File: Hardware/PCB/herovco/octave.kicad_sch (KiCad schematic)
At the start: 9 parts, among them SW1 SW_Rotary12

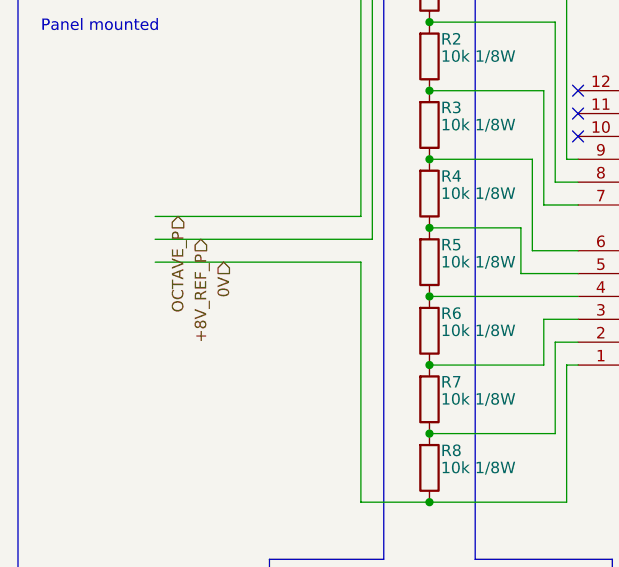
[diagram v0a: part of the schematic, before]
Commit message: Change pot symbols and fix orientation, other small tweaks
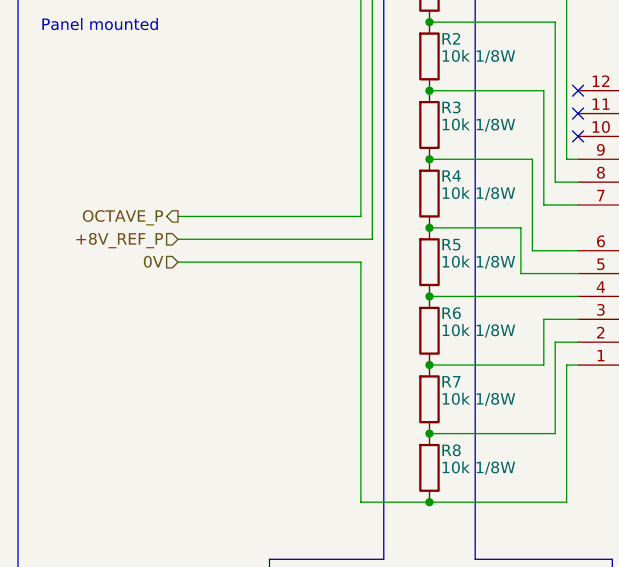
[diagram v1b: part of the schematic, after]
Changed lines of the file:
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@@
   (no_connect (at 147.32 82.55))
   (no_connect (at 147.32 77.47))
-  (wire (pts (xy 100.33 93.98) (xy 124.46 93.98))
+  (wire (pts (xy 102.87 93.98) (xy 124.46 93.98))
     (stroke (width 0) (type default) (color 0 0 0 0))
   )
@@
   )
   (polyline (pts (xy 125.73 129.54) (xy 113.03 129.54))
-    (stroke (width 0) (type default) (color 0 0 0 0))
+    (stroke (width 0) (type default) (color 194 0 194 1))
   )
   (wire (pts (xy 140.97 97.79) (xy 147.32 97.79))
@@
     (stroke (width 0) (type default) (color 0 0 0 0))
   )
-  (wire (pts (xy 100.33 91.44) (xy 123.19 91.44))
+  (wire (pts (xy 102.87 91.44) (xy 123.19 91.44))
     (stroke (width 0) (type default) (color 0 0 0 0))
   )
@@
   )
   (polyline (pts (xy 135.89 60.96) (xy 135.89 129.54))
-    (stroke (width 0) (type default) (color 0 0 0 0))
+    (stroke (width 0) (type default) (color 194 0 194 1))
   )
   (wire (pts (xy 140.97 92.71) (xy 140.97 97.79))
@@
   )
   (polyline (pts (xy 135.89 129.54) (xy 151.13 129.54))
-    (stroke (width 0) (type default) (color 0 0 0 0))
+    (stroke (width 0) (type default) (color 194 0 194 1))
   )
   (polyline (pts (xy 151.13 134.62) (xy 113.03 134.62))
-    (stroke (width 0) (type default) (color 0 0 0 0))
+    (stroke (width 0) (type default) (color 194 0 194 1))
   )
   (wire (pts (xy 143.51 77.47) (xy 143.51 90.17))
@@
     (stroke (width 0) (type default) (color 0 0 0 0))
   )
-  (wire (pts (xy 100.33 96.52) (xy 123.19 96.52))
+  (wire (pts (xy 102.87 96.52) (xy 123.19 96.52))
     (stroke (width 0) (type default) (color 0 0 0 0))
   )
@@
   )
   (polyline (pts (xy 125.73 60.96) (xy 125.73 129.54))
-    (stroke (width 0) (type default) (color 0 0 0 0))
+    (stroke (width 0) (type default) (color 194 0 194 1))
   )
   (polyline (pts (xy 113.03 129.54) (xy 113.03 134.62))
-    (stroke (width 0) (type default) (color 0 0 0 0))
+    (stroke (width 0) (type default) (color 194 0 194 1))
   )
   (polyline (pts (xy 85.09 140.97) (xy 179.07 140.97))
@@
   )
   (polyline (pts (xy 151.13 129.54) (xy 151.13 134.62))
-    (stroke (width 0) (type default) (color 0 0 0 0))
+    (stroke (width 0) (type default) (color 194 0 194 1))
   )
   (polyline (pts (xy 125.73 60.96) (xy 135.89 60.96))
-    (stroke (width 0) (type default) (color 0 0 0 0))
+    (stroke (width 0) (type default) (color 194 0 194 1))
   )
   (polyline (pts (xy 85.09 52.07) (xy 179.07 52.07))
@@
     (effects (font (size 1.27 1.27)) (justify left bottom))
   )
-  (hierarchical_label "0V" (shape input) (at 107.95 96.52 270)
+  (hierarchical_label "0V" (shape input) (at 102.87 96.52 180)
     (effects (font (size 1.27 1.27)) (justify right))
   )
-  (hierarchical_label "OCTAVE_P" (shape input) (at 102.87 91.44 270)
+  (hierarchical_label "OCTAVE_P" (shape output) (at 102.87 91.44 180)
     (effects (font (size 1.27 1.27)) (justify right))
   )
-  (hierarchical_label "+8V_REF_P" (shape input) (at 105.41 93.98 270)
+  (hierarchical_label "+8V_REF_P" (shape input) (at 102.87 93.98 180)
     (effects (font (size 1.27 1.27)) (justify right))
   )
-  (symbol (lib_id "Switch:SW_Rotary12") (at 157.48 92.71 180)
+  (symbol (lib_id "Switch:SW_Rotary12") (at 157.48 92.71 180) (unit 1)
     (in_bom yes) (on_board yes)
     (property "Reference" "SW1" (id 0) (at 160.02 71.755 0))
@@
     (pin "9")
   )
-  (symbol (lib_id "ao_symbols:R") (at 130.81 66.04 0) (mirror x)
+  (symbol (lib_id "ao_symbols:R") (at 130.81 66.04 0) (mirror x) (unit 1)
     (in_bom yes) (on_board yes)
     (property "Reference" "R1" (id 0) (at 132.08 64.135 0)
@@
     (pin "2")
   )
-  (symbol (lib_id "ao_symbols:R") (at 130.81 73.66 0) (mirror x)
+  (symbol (lib_id "ao_symbols:R") (at 130.81 73.66 0) (mirror x) (unit 1)
     (in_bom yes) (on_board yes)
     (property "Reference" "R2" (id 0) (at 132.08 71.755 0)
@@
     (pin "2")
   )
-  (symbol (lib_id "ao_symbols:R") (at 130.81 81.28 0) (mirror x)
+  (symbol (lib_id "ao_symbols:R") (at 130.81 81.28 0) (mirror x) (unit 1)
     (in_bom yes) (on_board yes)
     (property "Reference" "R3" (id 0) (at 132.08 79.375 0)
@@
     (pin "2")
   )
-  (symbol (lib_id "ao_symbols:R") (at 130.81 88.9 0) (mirror x)
+  (symbol (lib_id "ao_symbols:R") (at 130.81 88.9 0) (mirror x) (unit 1)
     (in_bom yes) (on_board yes)
     (property "Reference" "R4" (id 0) (at 132.08 86.995 0)
@@
     (pin "2")
   )
-  (symbol (lib_id "ao_symbols:R") (at 130.81 96.52 0) (mirror x)
+  (symbol (lib_id "ao_symbols:R") (at 130.81 96.52 0) (mirror x) (unit 1)
     (in_bom yes) (on_board yes)
     (property "Reference" "R5" (id 0) (at 132.08 94.615 0)
@@
     (pin "2")
   )
-  (symbol (lib_id "ao_symbols:R") (at 130.81 104.14 0) (mirror x)
+  (symbol (lib_id "ao_symbols:R") (at 130.81 104.14 0) (mirror x) (unit 1)
     (in_bom yes) (on_board yes)
     (property "Reference" "R6" (id 0) (at 132.08 102.235 0)
@@
     (pin "2")
   )
-  (symbol (lib_id "ao_symbols:R") (at 130.81 111.76 0) (mirror x)
+  (symbol (lib_id "ao_symbols:R") (at 130.81 111.76 0) (mirror x) (unit 1)
     (in_bom yes) (on_board yes)
     (property "Reference" "R7" (id 0) (at 132.08 109.855 0)
@@
     (pin "2")
   )
-  (symbol (lib_id "ao_symbols:R") (at 130.81 119.38 0) (mirror x)
+  (symbol (lib_id "ao_symbols:R") (at 130.81 119.38 0) (mirror x) (unit 1)
     (in_bom yes) (on_board yes)
     (property "Reference" "R8" (id 0) (at 132.08 117.475 0)

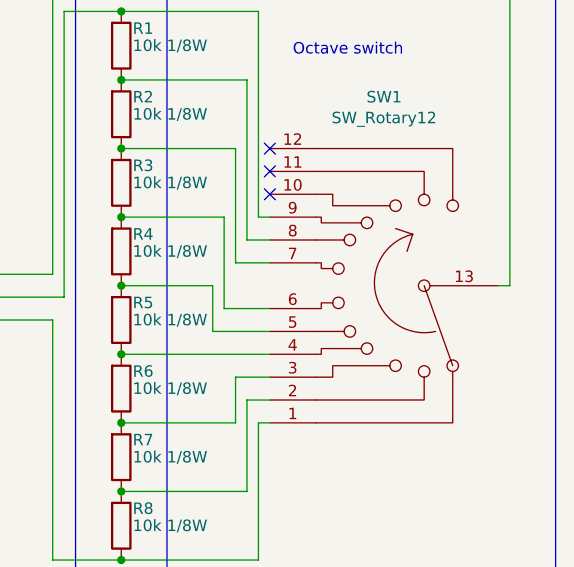
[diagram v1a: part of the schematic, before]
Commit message: Pre-breadboard updates
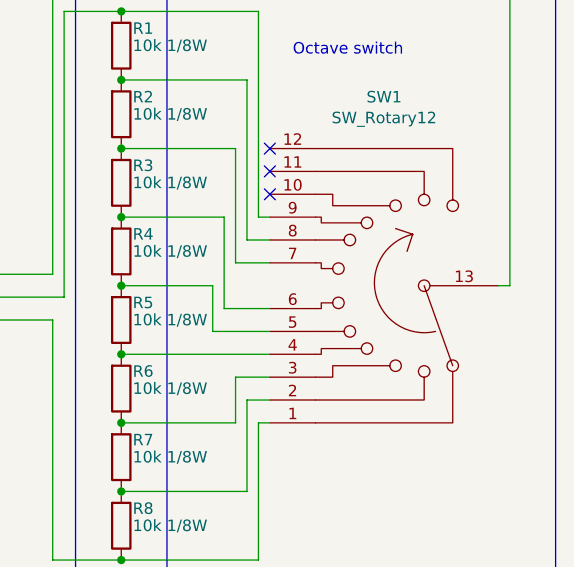
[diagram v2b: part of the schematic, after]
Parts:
- SW1: symbol Switch:SW_Rotary12 -> ao_symbols:SW_Rotary12; SKU (none) -> A-1893; Vendor (none) -> Tayda
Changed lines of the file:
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@@
     (comment 1 "or neighboring rights to this work. Published from United States.")
     (comment 2 "To the extent possible under law, Richard Holmes has waived all copyright and related ")
-    (comment 3 "Based mainly on Kassutronics VCO 3340")
+    (comment 3 "Partly based on designs by Kassutronics, Thomas Henry, and LMNC")
   )
   (junction (at 130.81 92.71) (diameter 0) (color 0 0 0 0)
@@
     (effects (font (size 1.27 1.27)) (justify right))
   )
-  (symbol (lib_id "Switch:SW_Rotary12") (at 157.48 92.71 180) (unit 1)
+  (symbol (lib_id "ao_symbols:SW_Rotary12") (at 157.48 92.71 180) (unit 1)
     (in_bom yes) (on_board yes)
     (property "Reference" "SW1" (id 0) (at 160.02 71.755 0))
@@
       (effects (font (size 1.27 1.27)) hide)
     )
+    (property "Vendor" "Tayda" (id 4) (at 157.48 92.71 0)
+      (effects (font (size 1.27 1.27)) hide)
+    )
+    (property "SKU" "A-1893" (id 5) (at 157.48 92.71 0)
+      (effects (font (size 1.27 1.27)) hide)
+    )

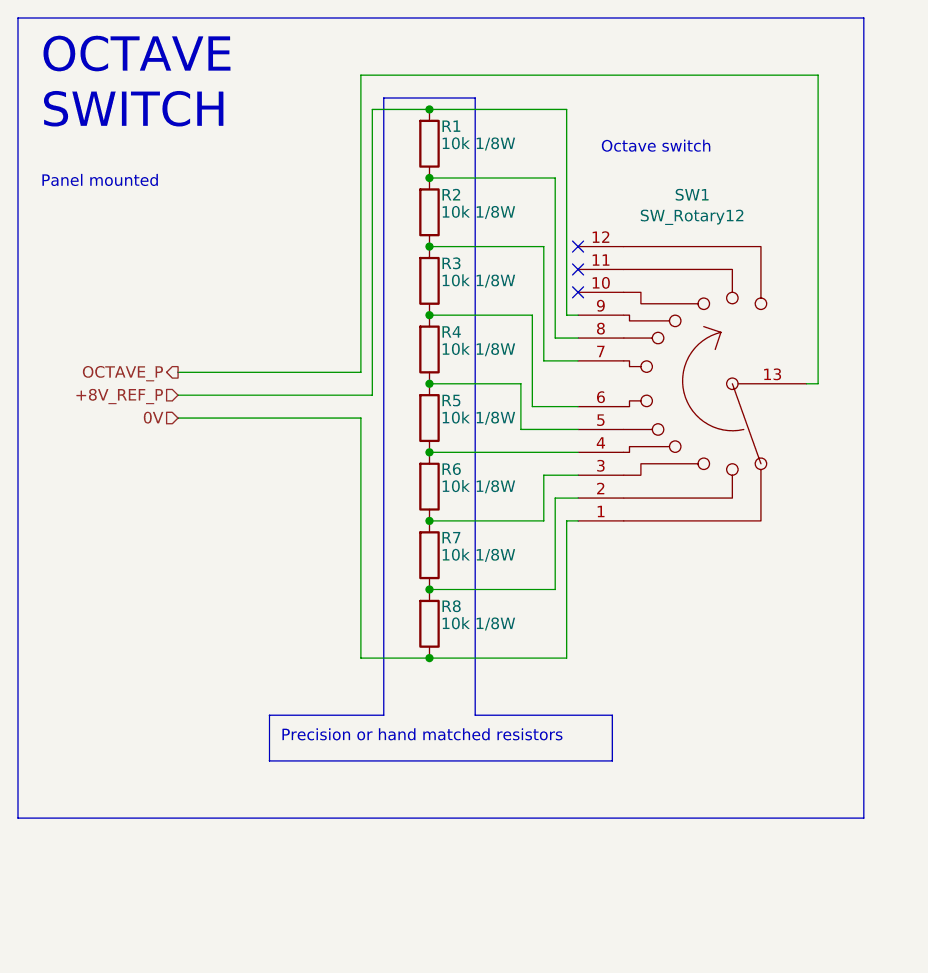
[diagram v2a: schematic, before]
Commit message: rm Zener, change adj ref to fixed and modify octave switch and fine tune accordingly
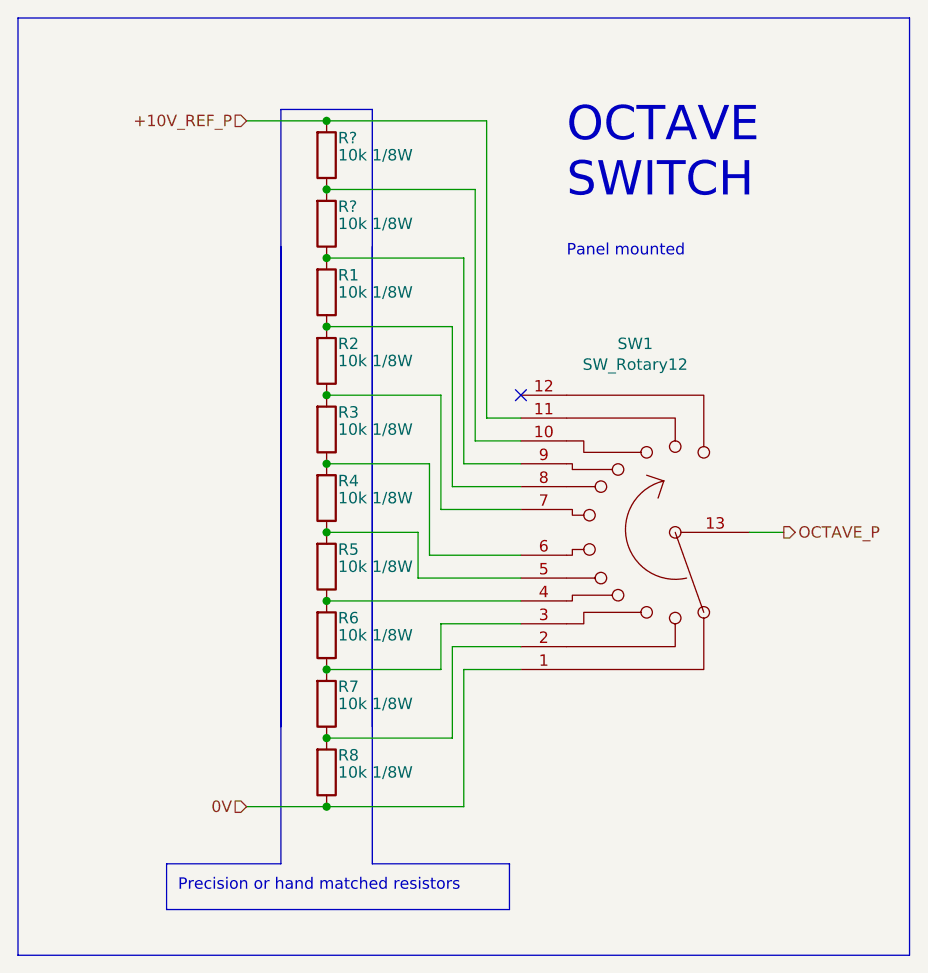
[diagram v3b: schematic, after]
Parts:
- added R? (x2): 10k 1/8W, ao_tht:R_Axial_DIN0207_L6.3mm_D2.5mm_P10.16mm_Horizontal, symbol ao_symbols:R
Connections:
- net at SW1.10: now also R?.1, R?.2
- net +10V_REF_P: now reaches SW1.11
- net +10V_REF_P: now also R?.2
- net +8V_REF_P: no longer names the net of R1.2, SW1.9
- net +8V_REF_P: now also R?.1
- no-connect marks 3 -> 1
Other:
- note removed: "Octave switch"
- moved on the sheet: R1, R2, R3, R4, R5, R6, R7, R8, SW1
